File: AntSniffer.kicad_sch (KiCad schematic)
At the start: 4 parts, among them CN1 X2026WRS-2X09D-LPSW, CN2 X2026WRS-2X09D-LPSW, J1 Conn_01x10_MountingPin

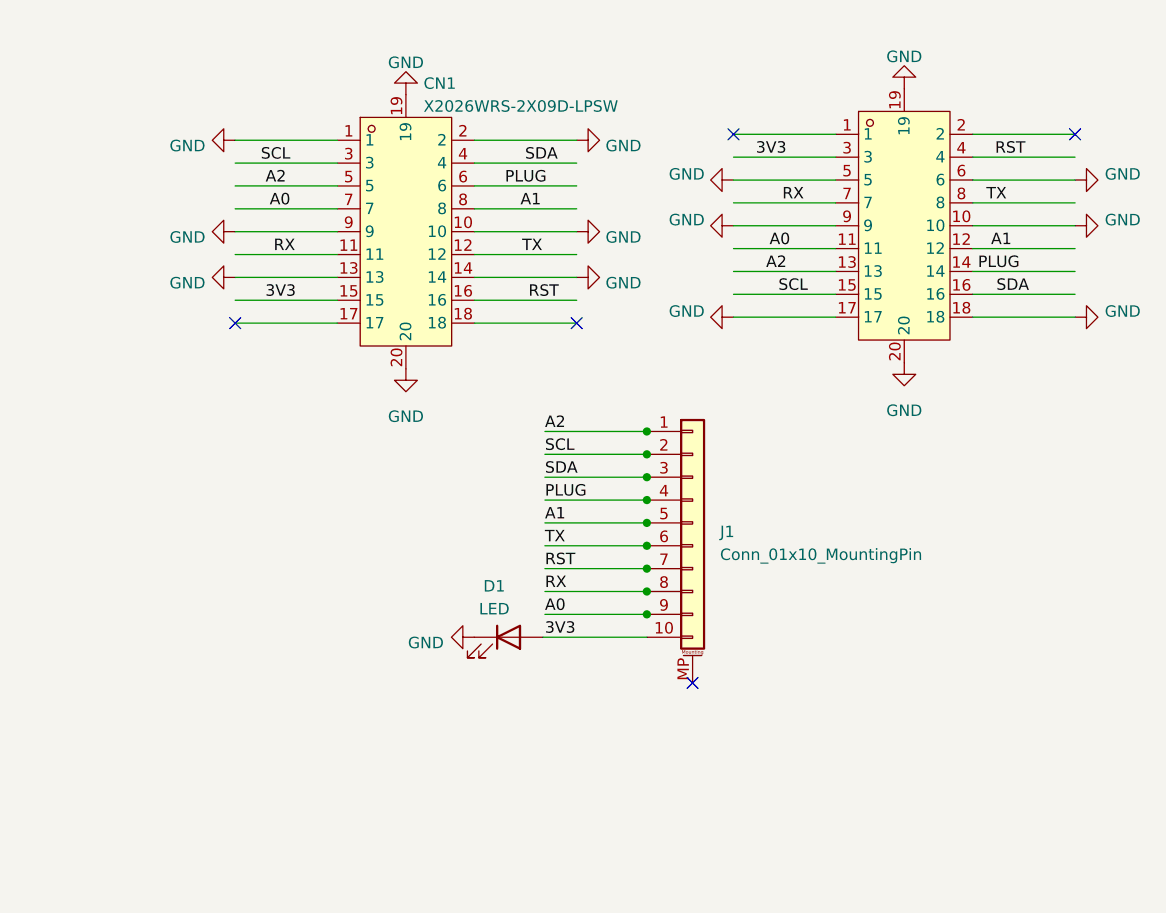
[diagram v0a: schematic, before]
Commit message: Release V2.1
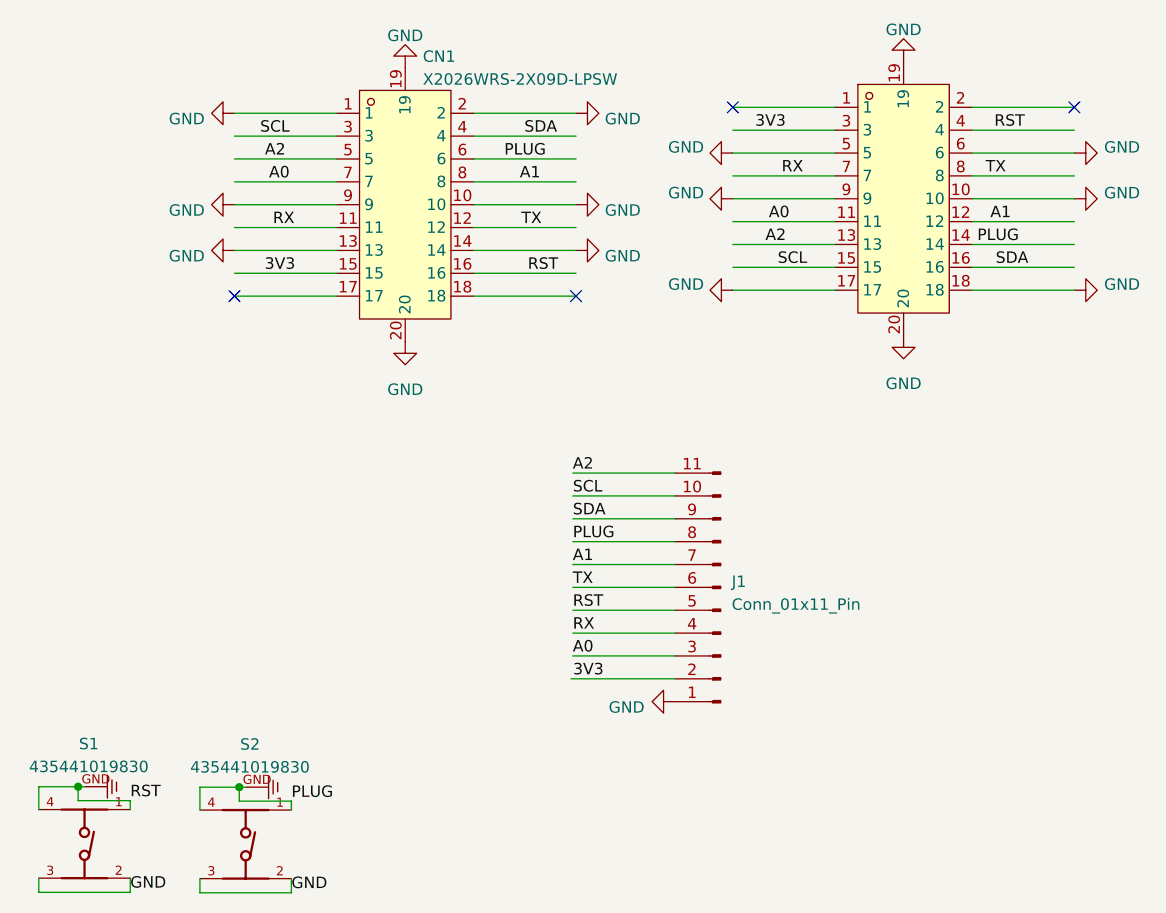
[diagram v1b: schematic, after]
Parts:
- removed D1: LED, LED_SMD:LED_0603_1608Metric, symbol Device:LED
- removed J1: Conn_01x10_MountingPin, Connector_PinHeader_2.54mm:PinHeader_1x10_P2.54mm_Vertical, symbol Connector_Generic_MountingPin:Conn_01x10_MountingPin
- added J1: Conn_01x11_Pin, Connector_PinHeader_2.54mm:PinHeader_1x11_P2.54mm_Vertical, symbol Connector:Conn_01x11_Pin
- added S1, S2: 435441019830, DOWNLOADED:435441019830, symbol 435441019830:435441019830
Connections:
- net 3V3: now also J1.2 (Pin_2)
- net A0: now also J1.3 (Pin_3)
- net A1: now also J1.7 (Pin_7)
- net A2: now also J1.11 (Pin_11)
- net GND: now also J1.1 (Pin_1), S1.2, S1.3, S2.2, S2.3
- net PLUG: now also J1.8 (Pin_8), S2.1, S2.4, S2.GND
- net RST: now also J1.5 (Pin_5), S1.1, S1.4, S1.GND
- net RX: now also J1.4 (Pin_4)
- net SCL: now also J1.10 (Pin_10)
- net SDA: now also J1.9 (Pin_9)
- net TX: now also J1.6 (Pin_6)
- no-connect marks 5 -> 4
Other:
- moved on the sheet: CN1
